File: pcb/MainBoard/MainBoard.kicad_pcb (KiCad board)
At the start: 2 copper layers, 47 parts, among them P1 Camera pot 1, P2 Camera pot 2, P3 Motor controller, P4 Motor battery, P5 Steering connector, P6 Arduino battery, SW1 OnOffDoubleSwitch, U1 arduino_mini, U2 notgate_74HCT04, U3 arduino_mini

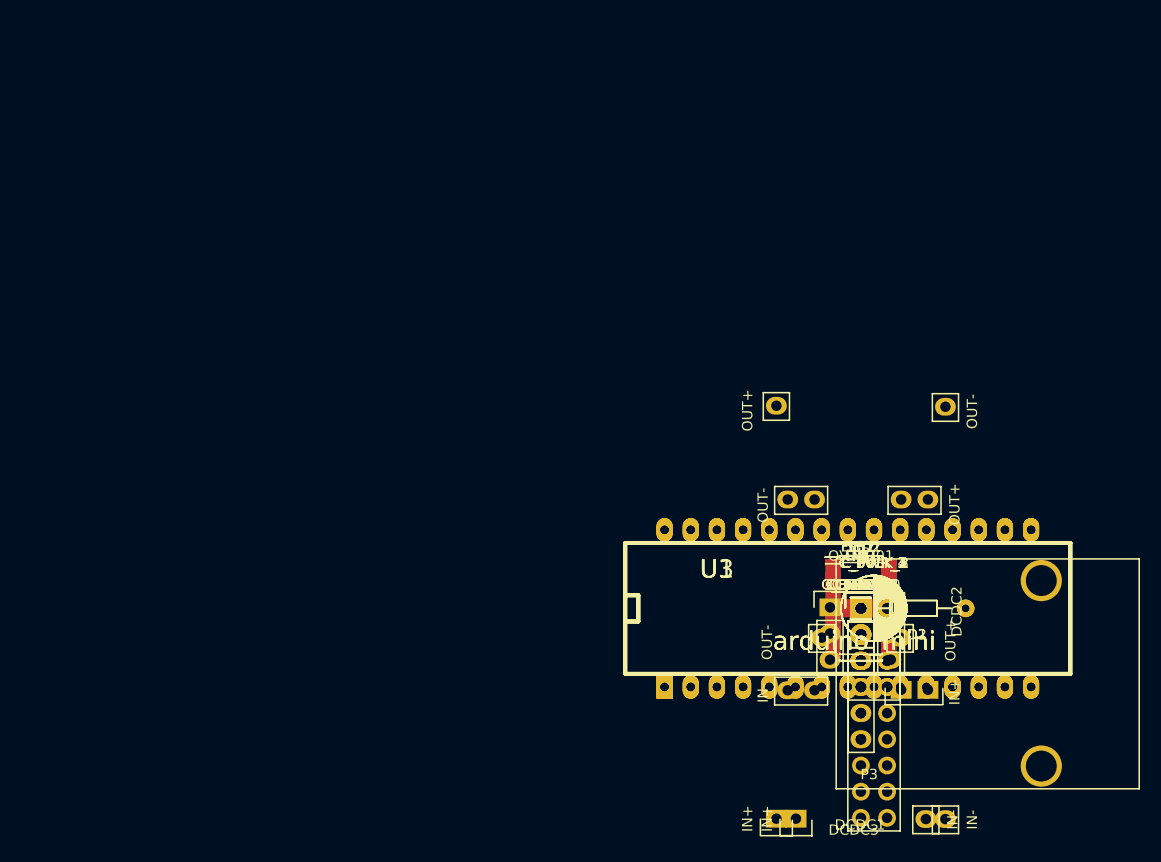
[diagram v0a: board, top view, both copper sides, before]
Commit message: PCB design finished
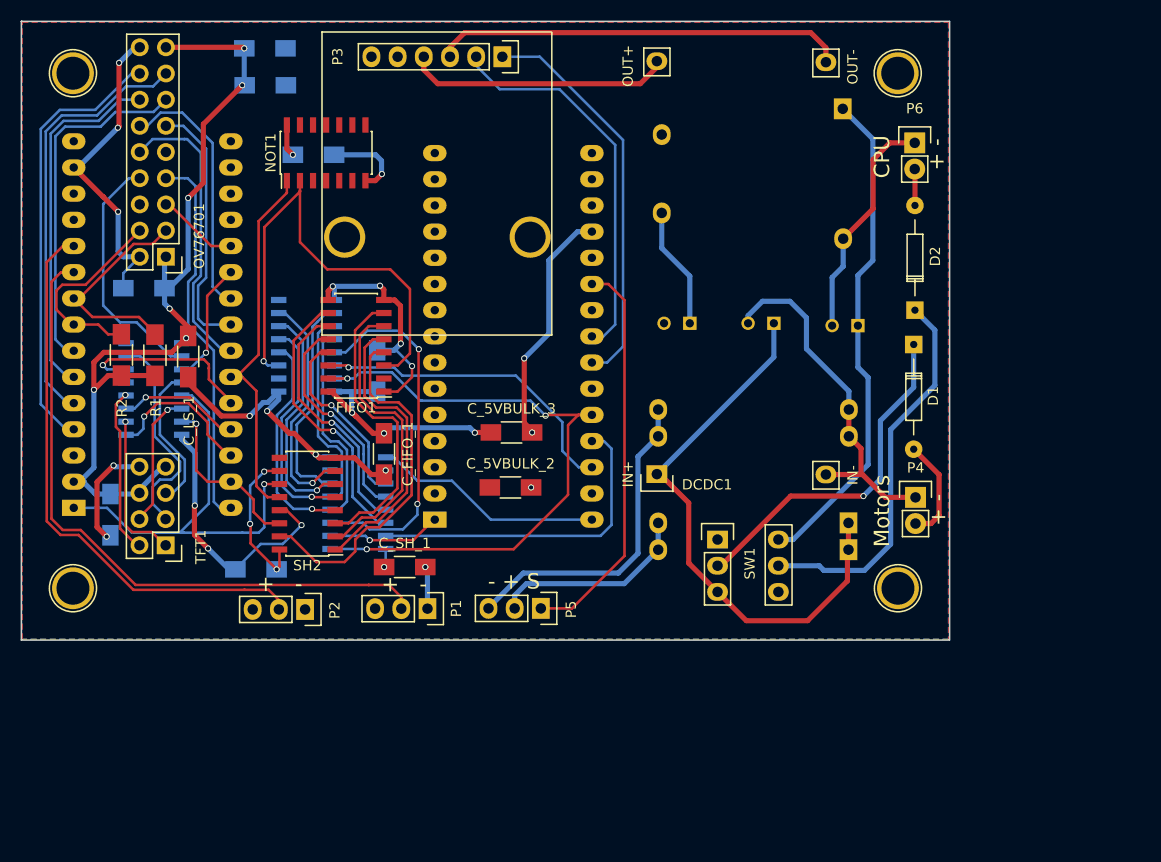
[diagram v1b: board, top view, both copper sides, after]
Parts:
- removed C_BULK_1, C_BULK_2, C_BULK_3: 10-100uF, Capacitors_ThroughHole:C_Radial_D6.3_L11.2_P2.5
- removed C_BULK_10, C_BULK_11, C_BULK_4, C_BULK_5, C_BULK_6, C_BULK_7, C_BULK_8, C_BULK_9: 10-100uF, Capacitors_SMD:C_1206_HandSoldering
- removed C_PWR_3, C_PWR_4: C, Capacitors_ThroughHole:C_Radial_D6.3_L11.2_P2.5
- removed U1, U3: arduino_mini, arduino:arduino_mini
- removed U2: notgate_74HCT04, Housings_SOIC:SOIC-14_3.9x8.7mm_Pitch1.27mm
- added ARD1: arduino_mini, arduino:arduino_mini, B.Cu at (79.8, 76.2)
- added ARD2: arduino_mini, arduino:arduino_mini, B.Cu at (114.8, 77.3)
- added C_3VBULK_1: 10-100uF, Capacitors_SMD:C_1206_HandSoldering, B.Cu at (90.7, 50.7)
- added C_3VBULK_2: 10-100uF, Capacitors_SMD:C_1206_HandSoldering, B.Cu at (90.7, 54.3)
- added C_5VBULK_1: 10-100uF, Capacitors_ThroughHole:C_Radial_D6.3_L11.2_P2.5, B.Cu at (131.9, 77.3)
- added C_5VBULK_2: 10-100uF, Capacitors_SMD:C_1206_HandSoldering, F.Cu at (114.5, 93.3)
- added C_5VBULK_3: 10-100uF, Capacitors_SMD:C_1206_HandSoldering, F.Cu at (114.6, 87.9)
- added NOT1: notgate_74HCT04, Housings_SOIC:SOIC-14_3.9x8.7mm_Pitch1.27mm, F.Cu at (96.6, 60.8)
- added REF**: 1pin, Connect:1pin, F.Cu at (152.1, 103.0)
- added REF**: 1pin, Connect:1pin, F.Cu at (152.1, 53.1)
- added REF**: 1pin, Connect:1pin, F.Cu at (72.1, 53.1)
- added REF**: 1pin, Connect:1pin, F.Cu at (72.1, 103.0)
- C_CAM_1, C_FIFO_2, C_NOT_1, C_PWR_1, C_PWR_2, C_SH_2, C_TFT_1, DCDC2, DCDC3, FIFO2, LS1, SH1: moved to B.Cu
- moved C_CAM_1 76.2 mm to (78.9, 73.9), turned to 180 degrees
- moved R2 75.8 mm to (76.8, 80.4), turned to 90 degrees
- moved OV76701 75.6 mm to (81.1, 70.9), turned to 180 degrees
- moved C_TFT_1 73.4 mm to (75.7, 95.9), turned to 270 degrees
- moved R1 72.8 mm to (80.0, 80.4), turned to 90 degrees
- moved LS1 71.8 mm to (79.9, 83.7), turned to 180 degrees
- moved C_LS_1 69.7 mm to (83.2, 80.6), turned to 270 degrees
- moved C_NOT_1 69.0 mm to (95.4, 61.0)
- moved TFT1 67.7 mm to (81.1, 98.9), turned to 180 degrees
- moved P3 63.8 mm to (113.7, 51.5), turned to 270 degrees
- moved FIFO2 59.5 mm to (94.7, 79.5)
- moved C_SH_2 58.8 mm to (89.8, 101.2), turned to 180 degrees
- moved FIFO1 55.2 mm to (99.5, 79.5), turned to 180 degrees
- moved SH2 54.7 mm to (94.8, 94.8), turned to 180 degrees
- moved P2 53.9 mm to (94.6, 105.1), turned to 270 degrees
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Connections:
- C_PWR_2 pad 1: Net-(C_PWR_1-Pad1) -> Net-(C_PWR_2-Pad1)
- C_PWR_2 pad 2: Net-(C_PWR_1-Pad2) -> Net-(C_PWR_2-Pad2)
- DCDC3 pad 1: Net-(C_PWR_3-Pad1) -> Net-(C_PWR_2-Pad1)
- DCDC3 pad 2: Net-(C_PWR_3-Pad2) -> Net-(C_PWR_2-Pad2)
- P6 pad 1: Net-(C_PWR_3-Pad2) -> Net-(C_PWR_2-Pad2)
- SW1 pad 6: Net-(C_PWR_3-Pad1) -> Net-(C_PWR_2-Pad1)
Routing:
- net GND: track 0.00 -> 160.9 mm, vias 0 -> 21
- net Net-(ARD1-Pad2): track 0.00 -> 85.5 mm, vias 0 -> 6
- net Net-(ARD1-Pad10): track 0.00 -> 64.8 mm
- net /SectionCommBuffer/FIFO_POP: track 0.00 -> 63.7 mm, vias 0 -> 3
- net +5V: track 0.00 -> 60.2 mm, vias 0 -> 8
- net Net-(ARD1-Pad11): track 0.00 -> 56.0 mm
- net Net-(C_PWR_1-Pad1): track 0.00 -> 54.4 mm
- net Net-(C_PWR_2-Pad1): track 0.00 -> 48.5 mm
- net Net-(FIFO1-Pad3): track 0.00 -> 47.4 mm, vias 0 -> 1
- net /Sheet57F22415/Pixel_D0: track 0.00 -> 42.7 mm
- net /Sheet57F22415/Pixel_D1: track 0.00 -> 41.8 mm
- net /Sheet57F22415/SPI_CLOCK: track 0.00 -> 41.6 mm, vias 0 -> 1
- net Net-(DCDC1-Pad4): track 0.00 -> 40.0 mm
- net /SectionMainControl/STEERING: track 0.00 -> 38.8 mm
- net /SectionMainControl/FORWARD: track 0.00 -> 38.8 mm
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- added copper zone on F.Cu, net +5V
- added copper zone on B.Cu, net GND
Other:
- board outline added: 90 x 60 mm
- board text added: "+ -"
- board text added: "- + S"
- board text added: "CPU"
- board text added: "Motors"
